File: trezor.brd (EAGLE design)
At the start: 50 x 26.7 mm, 27 parts, among them IC1 MCP1703CB, Q2 16MHz, U1 STM32F205RET6, U2 USB, U3 DISPLAY

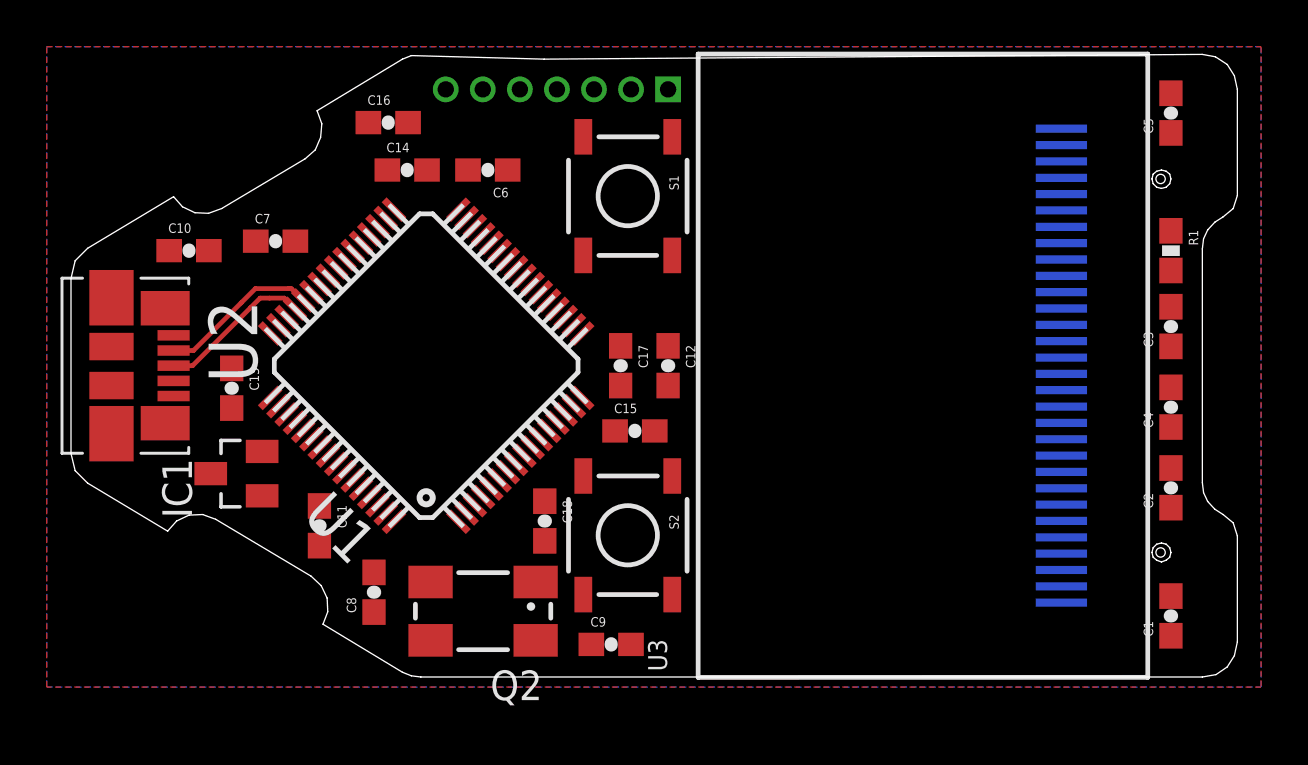
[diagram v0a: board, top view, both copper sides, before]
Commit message: WIP
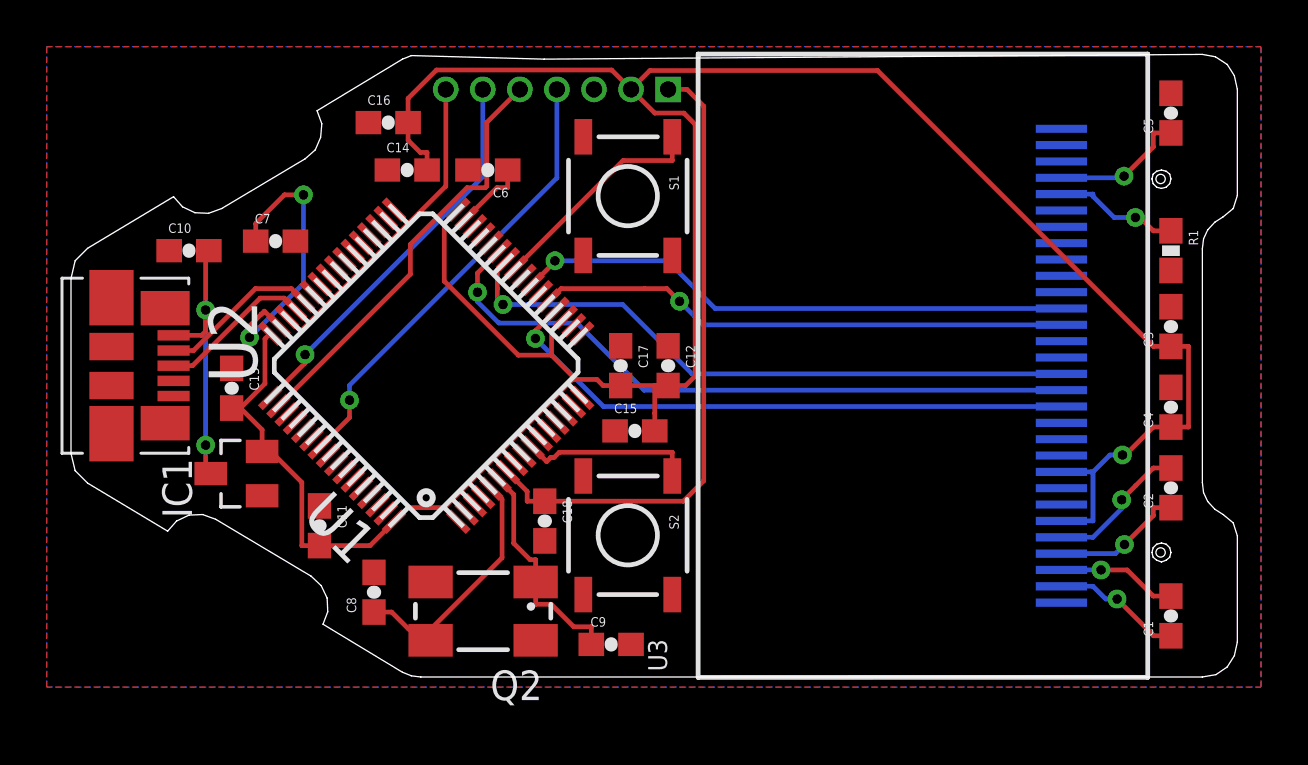
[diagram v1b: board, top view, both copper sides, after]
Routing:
- net +3V3: track 0.00 -> 118.1 mm, vias 0 -> 1
- net N$7: track 0.00 -> 29.1 mm, vias 0 -> 1
- net N$2: track 0.00 -> 27.4 mm
- net N$3: track 0.00 -> 27.4 mm, vias 0 -> 1
- net N$16: track 0.00 -> 25.4 mm, vias 0 -> 1
- net N$1: track 0.00 -> 23.9 mm, vias 0 -> 1
- net N$5: track 0.00 -> 22.8 mm, vias 0 -> 1
- net N$14: track 0.00 -> 19.5 mm, vias 0 -> 1
- net N$18: track 0.00 -> 18.3 mm
- net N$17: track 0.00 -> 17.0 mm, vias 0 -> 1
- net N$15: track 0.00 -> 13.8 mm
- net N$8: track 0.00 -> 12.6 mm, vias 0 -> 2
- net +5V: track 0.00 -> 12.2 mm, vias 0 -> 2
- net XTAL2: track 0.00 -> 10.7 mm
- net XTAL1: track 0.00 -> 9.62 mm
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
